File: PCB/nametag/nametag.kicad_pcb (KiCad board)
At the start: 4 copper layers, 59.2 x 29.2 mm, 56 parts, among them J1 USB_C_Receptacle_USB2.0_14P, J3 Conn_02x03_Odd_Even, Q1 NXV55UN, U1 MIC550x, U2 AVR64DU32, U3 23K640, U4 MCP9700x-ETT, U5 SN74LV1T125DBV, U6 SN74LV1T125DBV

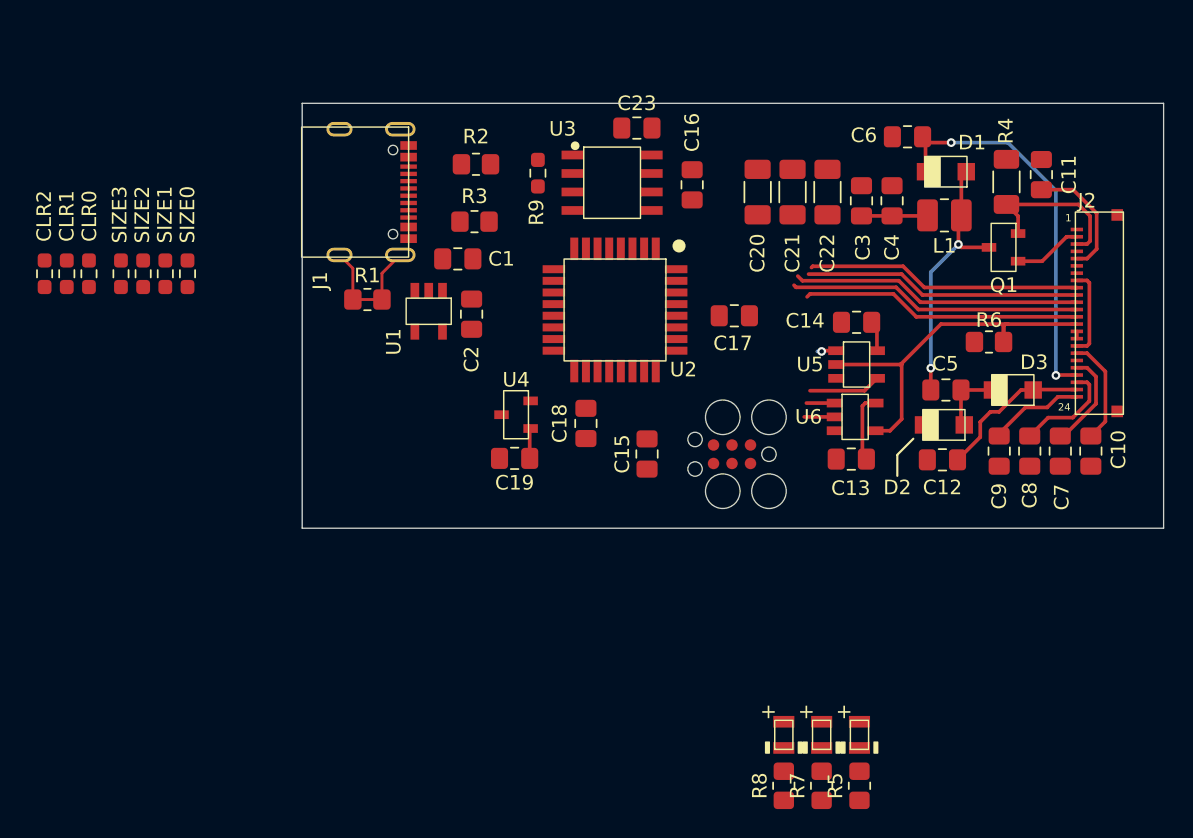
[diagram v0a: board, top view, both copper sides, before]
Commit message: PCB files. BOM. Step model.
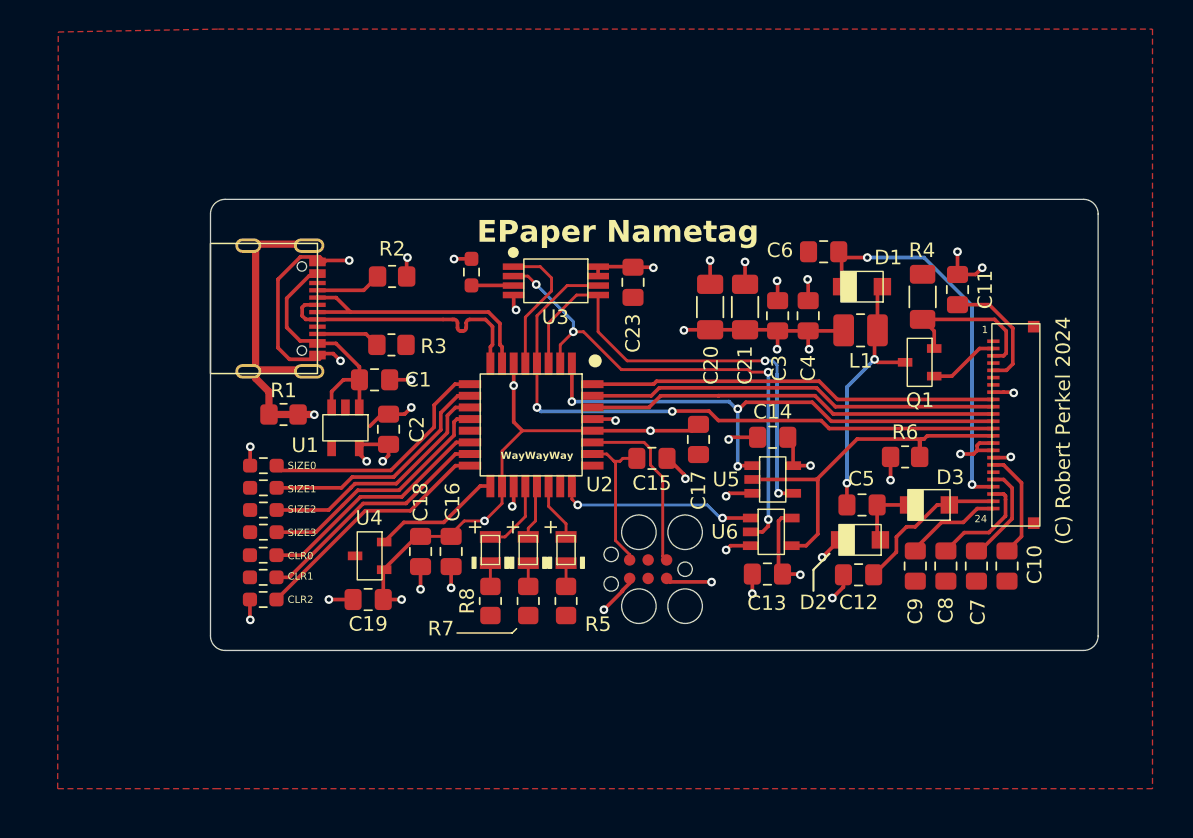
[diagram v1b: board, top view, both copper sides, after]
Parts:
- removed C22: 10uF, Capacitor_SMD:C_1206_3216Metric_Pad1.33x1.80mm_HandSolder
- U3: footprint StandardPackages_Custom:SOIC-8 -> Microchip:TSSOP-8 (ST)
- moved C16 30.2 mm to (186.0, 113.7)
- moved CLR2 27.0 mm to (173.1, 117.0), turned to 0 degrees
- moved CLR1 24.9 mm to (173.1, 115.5), turned to 0 degrees
- moved R5 23.8 mm to (193.9, 117.1)
- moved R7 23.8 mm to (191.3, 117.1)
- moved R8 23.8 mm to (188.7, 117.1)
- moved D4 23.8 mm to (193.9, 113.6)
- moved D5 23.8 mm to (191.3, 113.6)
- moved D6 23.8 mm to (188.7, 113.6)
- moved CLR0 22.7 mm to (173.1, 114.0), turned to 0 degrees
- moved SIZE3 20.3 mm to (173.1, 112.4), turned to 0 degrees
- moved SIZE2 18.2 mm to (173.1, 110.8), turned to 0 degrees
- moved SIZE1 16.2 mm to (173.1, 109.3), turned to 0 degrees
- moved C18 14.4 mm to (183.9, 113.7)
- moved SIZE0 14.2 mm to (173.1, 107.8), turned to 0 degrees
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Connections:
- U2 pad 1: ~{DISP_MISO_EN} -> ~{DISP_CS}
- U2 pad 23: ~{FLASH_CS} -> unconnected-(U2-PF3-Pad23)
- U2 pad 24: unconnected-(U2-PF4-Pad24) -> ~{DISP_MISO_EN}
- U2 pad 5: ~{DISP_CS} -> ~{FLASH_CS}
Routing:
- net GND: track 15.1 -> 86.1 mm, vias 0 -> 31
- net +3.3V: track 14.0 -> 76.4 mm, vias 0 -> 15
- net MOSI: track 2.10 -> 35.1 mm, vias 0 -> 4
- net MISO: track 4.95 -> 32.6 mm, vias 0 -> 2
- net SCLK: track 19.3 -> 43.3 mm, vias 0 -> 2
- net /D+: track 0.01 -> 18.9 mm
- net /D-: track 0.01 -> 18.4 mm
- net +5V: track 0.00 -> 17.3 mm
- net Net-(U2-PD6): track 0.00 -> 17.1 mm
- net Net-(U2-PD2): track 0.00 -> 17.0 mm
- net Net-(U2-PD1): track 0.00 -> 16.9 mm
- net Net-(U2-PD5): track 0.00 -> 16.8 mm
- net Net-(U2-PC3): track 0.00 -> 16.8 mm
- net Net-(U2-PD0): track 0.00 -> 16.6 mm
- net Net-(U2-PD4): track 0.00 -> 16.5 mm
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- added copper zone on In2.Cu, net +3.3V
- added copper zone on F.Cu, net GND
- added copper zone on In1.Cu, net GND
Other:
- board size 59.2 x 29.2 mm -> 61 x 31 mm
- board text added: "${REVISION}"
- board text added: "${TITLE}"
- board text added: "${TITLE} (C) Robert Perkel 2024 Revision ${REVISION} ${ISSUE_DATE}"
- board text added: "(C) Robert Perkel 2024"
- board text added: "WayWayWay"
